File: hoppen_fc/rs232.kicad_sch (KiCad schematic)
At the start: 7 parts, among them U12 SP3223

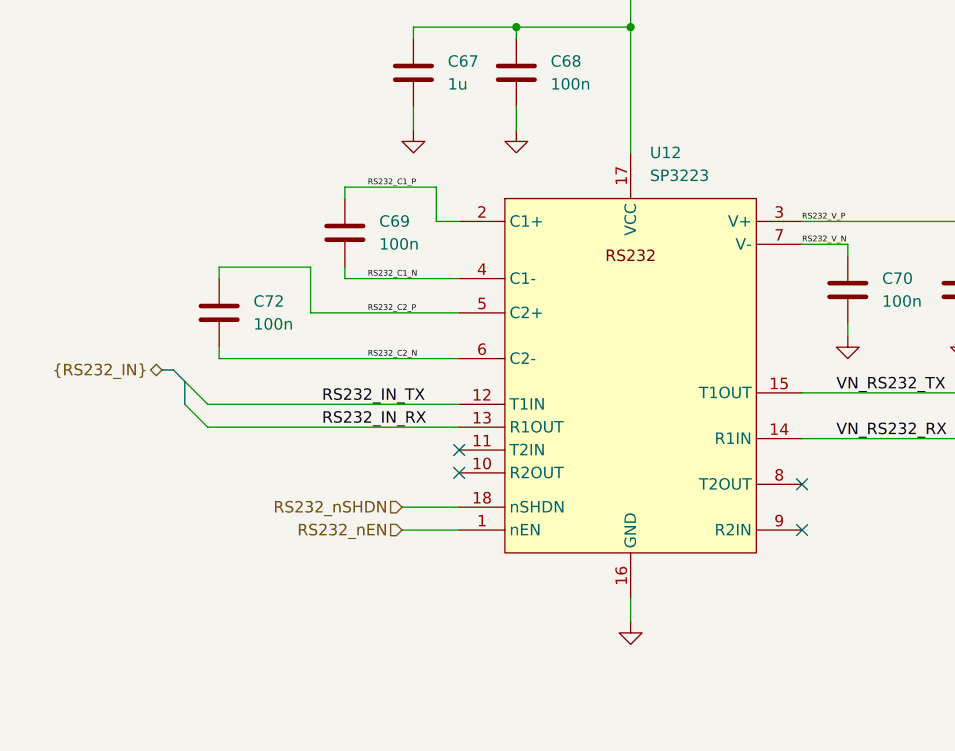
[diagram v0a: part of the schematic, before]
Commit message: ready for routing?
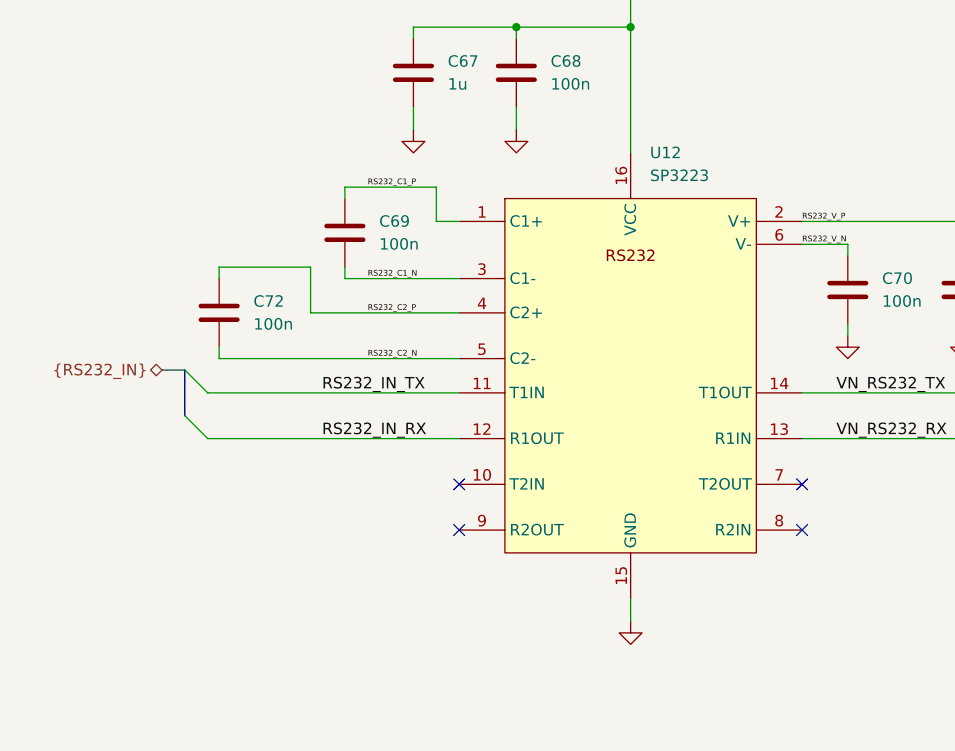
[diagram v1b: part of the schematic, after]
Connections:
- net RS232_nEN is gone; now on net RS232_C1_P: U12.1 (C1+)
- net +3V3: now also U12.16 (VCC); no longer U12.17 (VCC)
- net GND: now also U12.15 (GND); no longer U12.16 (GND)
- net RS232_C1_N: now also U12.3 (C1-); no longer U12.4 (C1-)
- net RS232_C1_P: no longer U12.2 (C1+)
- net RS232_C2_N: now also U12.5 (C2-); no longer U12.6 (C2-)
- net RS232_C2_P: now also U12.4 (C2+); no longer U12.5 (C2+)
- net RS232_IN_RX: now also U12.12 (R1OUT); no longer U12.13 (R1OUT)
- net RS232_IN_TX: now also U12.11 (T1IN); no longer U12.12 (T1IN)
- net RS232_V_N: now also U12.6 (V-); no longer U12.7 (V-)
- net RS232_V_P: now also U12.2 (V+); no longer U12.3 (V+)
- net VN_RS232_RX: now also U12.13 (R1IN); no longer U12.14 (R1IN)
- net VN_RS232_TX: now also U12.14 (T1OUT); no longer U12.15 (T1OUT)
- removed net RS232_nSHDN: U12.18 (nSHDN)
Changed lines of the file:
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@@
 	)
 	(no_connect
-		(at 120.65 106.68)
+		(at 120.65 110.49)
 	)
 	(no_connect
-		(at 120.65 109.22)
+		(at 120.65 115.57)
 	)
 	(no_connect
@@
 	)
 	(bus_entry
-		(at 90.17 99.06)
+		(at 90.17 97.79)
 		(size 2.54 2.54)
 		(stroke
@@
 	)
 	(bus_entry
-		(at 90.17 101.6)
+		(at 90.17 102.87)
 		(size 2.54 2.54)
 		(stroke
@@
 	(bus
 		(pts
-			(xy 87.63 97.79) (xy 88.9 97.79)
+			(xy 87.63 97.79) (xy 90.17 97.79)
 		)
 		(stroke
@@
 	(wire
 		(pts
-			(xy 92.71 101.6) (xy 120.65 101.6)
-		)
-		(stroke
-			(width 0)
-			(type default)
-		)
-	)
-	(wire
-		(pts
-			(xy 114.3 113.03) (xy 120.65 113.03)
+			(xy 92.71 100.33) (xy 120.65 100.33)
 		)
 		(stroke
@@
 	(wire
 		(pts
-			(xy 114.3 115.57) (xy 120.65 115.57)
-		)
-		(stroke
-			(width 0)
-			(type default)
-		)
-	)
-	(wire
-		(pts
 			(xy 176.53 81.28) (xy 176.53 85.09)
 		)
@@
 		)
 	)
+	(wire
+		(pts
+			(xy 107.95 77.47) (xy 118.11 77.47)
+		)
+		(stroke
+			(width 0)
+			(type default)
+		)
+	)
+	(wire
+		(pts
+			(xy 139.7 59.69) (xy 139.7 73.66)
+		)
+		(stroke
+			(width 0)
+			(type default)
+		)
+	)
+	(wire
+		(pts
+			(xy 107.95 78.74) (xy 107.95 77.47)
+		)
+		(stroke
+			(width 0)
+			(type default)
+		)
+	)
+	(wire
+		(pts
+			(xy 127 59.69) (xy 139.7 59.69)
+		)
+		(stroke
+			(width 0)
+			(type default)
+		)
+	)
+	(wire
+		(pts
+			(xy 127 68.58) (xy 127 71.12)
+		)
+		(stroke
+			(width 0)
+			(type default)
+		)
+	)
 	(bus
 		(pts
-			(xy 90.17 99.06) (xy 88.9 97.79)
-		)
-		(stroke
-			(width 0)
-			(type default)
-		)
-	)
-	(wire
-		(pts
-			(xy 107.95 77.47) (xy 118.11 77.47)
-		)
-		(stroke
-			(width 0)
-			(type default)
-		)
-	)
-	(wire
-		(pts
-			(xy 139.7 59.69) (xy 139.7 73.66)
-		)
-		(stroke
-			(width 0)
-			(type default)
-		)
-	)
-	(wire
-		(pts
-			(xy 107.95 78.74) (xy 107.95 77.47)
-		)
-		(stroke
-			(width 0)
-			(type default)
-		)
-	)
-	(wire
-		(pts
-			(xy 127 59.69) (xy 139.7 59.69)
-		)
-		(stroke
-			(width 0)
-			(type default)
-		)
-	)
-	(wire
-		(pts
-			(xy 127 68.58) (xy 127 71.12)
+			(xy 181.61 97.79) (xy 181.61 102.87)
+		)
+		(stroke
+			(width 0)
+			(type default)
+		)
+	)
+	(wire
+		(pts
+			(xy 115.57 59.69) (xy 127 59.69)
+		)
+		(stroke
+			(width 0)
+			(type default)
+		)
+	)
+	(wire
+		(pts
+			(xy 158.75 105.41) (xy 179.07 105.41)
+		)
+		(stroke
+			(width 0)
+			(type default)
+		)
+	)
+	(wire
+		(pts
+			(xy 93.98 86.36) (xy 93.98 87.63)
 		)
 		(stroke
@@
 	(bus
 		(pts
-			(xy 181.61 97.79) (xy 181.61 102.87)
-		)
-		(stroke
-			(width 0)
-			(type default)
-		)
-	)
-	(wire
-		(pts
-			(xy 115.57 59.69) (xy 127 59.69)
-		)
-		(stroke
-			(width 0)
-			(type default)
-		)
-	)
-	(wire
-		(pts
-			(xy 158.75 105.41) (xy 179.07 105.41)
-		)
-		(stroke
-			(width 0)
-			(type default)
-		)
-	)
-	(wire
-		(pts
-			(xy 93.98 86.36) (xy 93.98 87.63)
-		)
-		(stroke
-			(width 0)
-			(type default)
-		)
-	)
-	(bus
-		(pts
-			(xy 90.17 99.06) (xy 90.17 101.6)
+			(xy 90.17 97.79) (xy 90.17 102.87)
 		)
 		(stroke
@@
 	(wire
 		(pts
-			(xy 92.71 104.14) (xy 120.65 104.14)
+			(xy 92.71 105.41) (xy 120.65 105.41)
 		)
 		(stroke
@@
 	)
 	(label "RS232_IN_RX"
-		(at 105.41 104.14 0)
+		(at 105.41 105.41 0)
 		(effects
 			(font
@@
 	)
 	(label "RS232_IN_TX"
-		(at 105.41 101.6 0)
+		(at 105.41 100.33 0)
 		(effects
 			(font
@@
 			)
 			(justify left bottom)
-		)
-	)
-	(hierarchical_label "RS232_nSHDN"
-		(shape input)
-		(at 114.3 113.03 180)
-		(effects
-			(font
-				(size 1.27 1.27)
-			)
-			(justify right)
 		)
 	)
@@
 			)
 			(justify left)
-		)
-	)
-	(hierarchical_label "RS232_nEN"
-		(shape input)
-		(at 114.3 115.57 180)
-		(effects
-			(font
-				(size 1.27 1.27)
-			)
-			(justify right)
 		)
 	)
@@
 		(pin "6"
 		)
-		(pin "18"
-		)
 		(pin "1"
 		)
-		(pin "17"
-		)
 		(pin "10"
